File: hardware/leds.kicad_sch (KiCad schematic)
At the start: 4 parts, among them J21 USB_C_Receptacle_USB2.0_16P

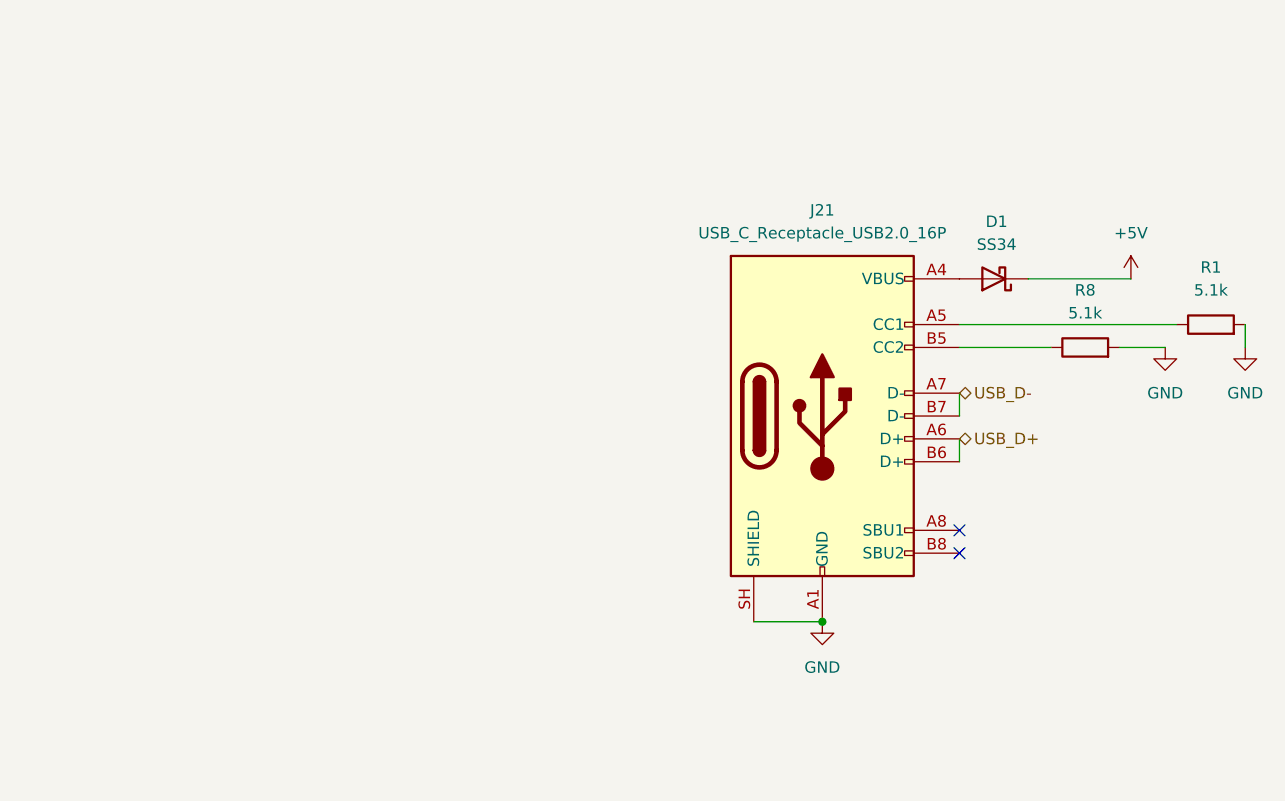
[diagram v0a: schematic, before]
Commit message: make the schematics
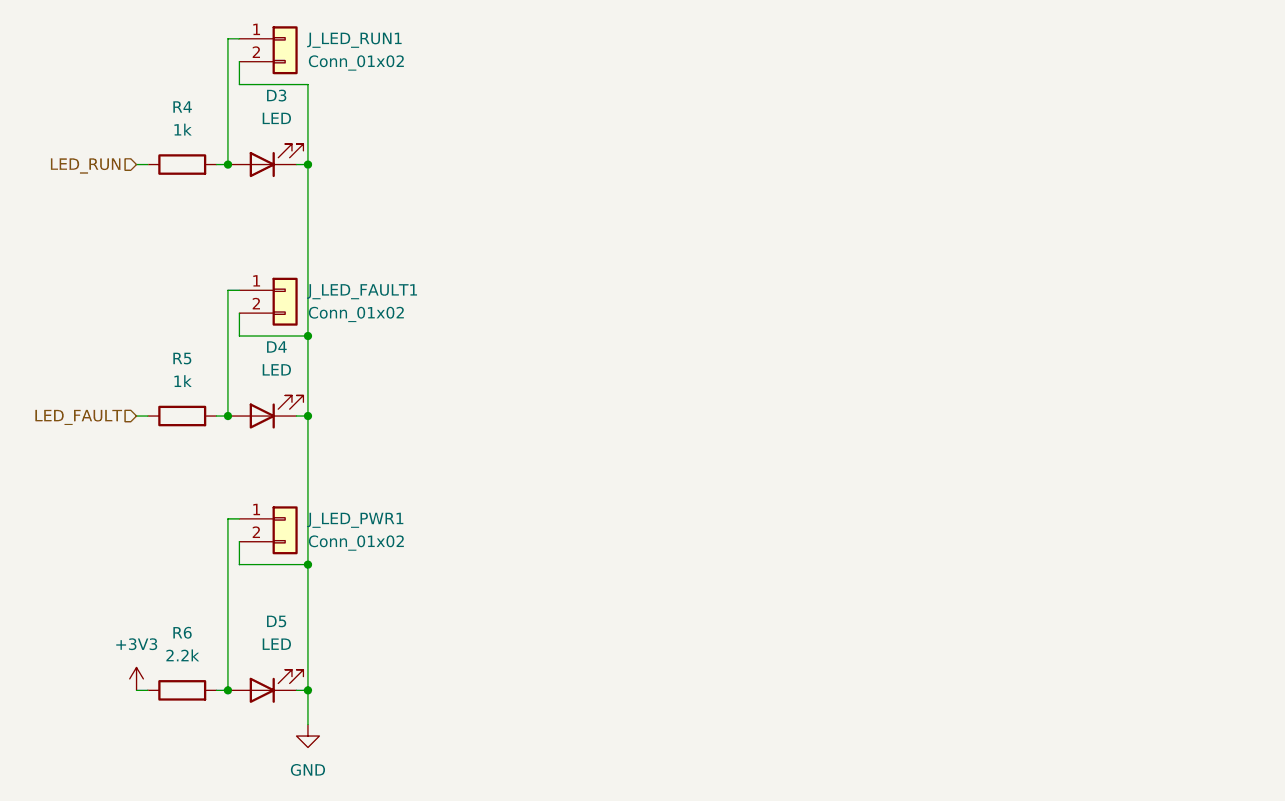
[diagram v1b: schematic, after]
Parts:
- removed D1: SS34, Diode_SMD:D_SMA, symbol Device:D_Schottky
- removed J21: USB_C_Receptacle_USB2.0_16P, symbol Connector:USB_C_Receptacle_USB2.0_16P
- removed R1, R8: 5.1k, symbol Device:R
- added D3, D4, D5: LED, symbol Device:LED
- added J_LED_FAULT1, J_LED_PWR1, J_LED_RUN1: Conn_01x02, symbol Connector_Generic:Conn_01x02
- added R4, R5: 1k, symbol Device:R
- added R6: 2.2k, symbol Device:R
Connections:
- net GND: now also D3.1 (K), D4.1 (K), D5.1 (K), J_LED_FAULT1.2 (Pin_2), J_LED_PWR1.2 (Pin_2), J_LED_RUN1.2 (Pin_2)
- new net: D4.2 (A), J_LED_FAULT1.1 (Pin_1), R5.2
- new net: D3.2 (A), J_LED_RUN1.1 (Pin_1), R4.2
- new net: D5.2 (A), J_LED_PWR1.1 (Pin_1), R6.2
- new net +3V3: R6.1
- new net LED_FAULT: R5.1
- new net LED_RUN: R4.1
- no-connect marks 2 -> 0

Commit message: place the stuff on the pcb
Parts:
- D3, D4, D5: footprint (none) -> LED_SMD:LED_2512_6332Metric
- J_LED_FAULT1, J_LED_PWR1, J_LED_RUN1: footprint (none) -> Connector_JST:JST_PH_B2B-PH-K_1x02_P2.00mm_Vertical
- R4, R5, R6: footprint (none) -> PCM_JLCPCB:R_0603
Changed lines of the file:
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@@
 			)
 		)
-		(property "Footprint" ""
+		(property "Footprint" "LED_SMD:LED_2512_6332Metric"
 			(at 53.34 74.93 0)
 			(hide yes)
@@
 			)
 		)
-		(property "Footprint" ""
+		(property "Footprint" "Connector_JST:JST_PH_B2B-PH-K_1x02_P2.00mm_Vertical"
 			(at 55.88 60.96 0)
 			(hide yes)
@@
 			)
 		)
-		(property "Footprint" ""
+		(property "Footprint" "PCM_JLCPCB:R_0603"
 			(at 44.45 76.708 90)
 			(hide yes)
@@
 			)
 		)
-		(property "Footprint" ""
+		(property "Footprint" "PCM_JLCPCB:R_0603"
 			(at 44.45 48.768 90)
 			(hide yes)
@@
 			)
 		)
-		(property "Footprint" ""
+		(property "Footprint" "PCM_JLCPCB:R_0603"
 			(at 44.45 107.188 90)
 			(hide yes)
@@
 			)
 		)
-		(property "Footprint" ""
+		(property "Footprint" "Connector_JST:JST_PH_B2B-PH-K_1x02_P2.00mm_Vertical"
 			(at 55.88 33.02 0)
 			(hide yes)
@@
 			)
 		)
-		(property "Footprint" ""
+		(property "Footprint" "LED_SMD:LED_2512_6332Metric"
 			(at 53.34 46.99 0)
 			(hide yes)
@@
 			)
 		)
-		(property "Footprint" ""
+		(property "Footprint" "LED_SMD:LED_2512_6332Metric"
 			(at 53.34 105.41 0)
 			(hide yes)
@@
 			)
 		)
-		(property "Footprint" ""
+		(property "Footprint" "Connector_JST:JST_PH_B2B-PH-K_1x02_P2.00mm_Vertical"
 			(at 55.88 86.36 0)
 			(hide yes)

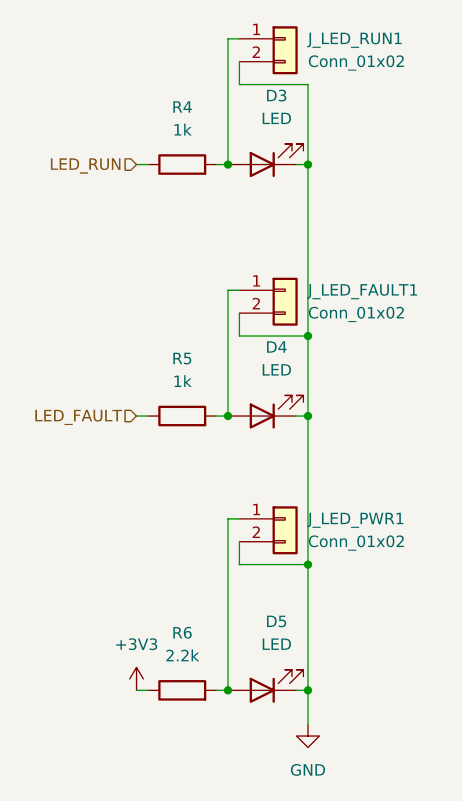
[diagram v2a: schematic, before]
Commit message: route
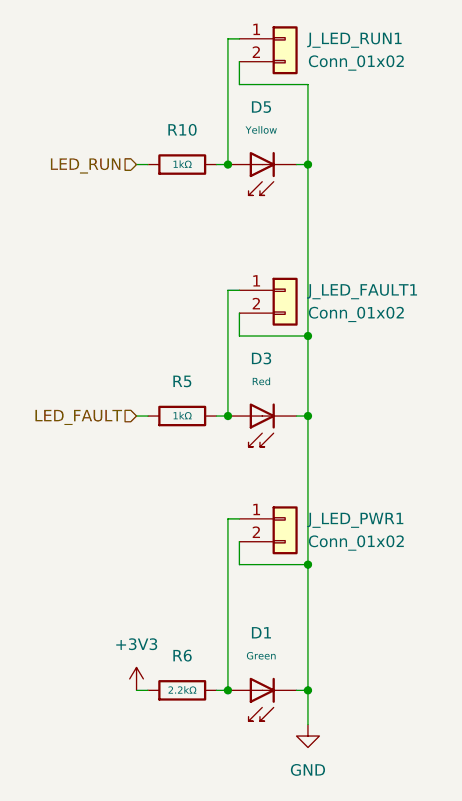
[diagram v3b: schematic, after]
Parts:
- removed D3, D4, D5: LED, LED_SMD:LED_2512_6332Metric, symbol Device:LED
- removed R4, R5: 1k, PCM_JLCPCB:R_0603, symbol Device:R
- removed R6: 2.2k, PCM_JLCPCB:R_0603, symbol Device:R
- added D1: Green, PCM_JLCPCB:D_0805, symbol PCM_JLCPCB-Diodes:LED,0805,Green
- added D3: Red, PCM_JLCPCB:D_0603, symbol PCM_JLCPCB-Diodes:LED,0603,Red
- added D5: Yellow, PCM_JLCPCB:D_0603, symbol PCM_JLCPCB-Diodes:LED,0603,Yellow
- added R10, R5: 1kΩ, PCM_JLCPCB:R_0603, symbol PCM_JLCPCB-Resistors:0603,1kΩ
- added R6: 2.2kΩ, PCM_JLCPCB:R_0603, symbol PCM_JLCPCB-Resistors:0603,2.2kΩ
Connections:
- net +3V3: now also R6.1
- net GND: now also D1.1, D3.1, D5.1
- net LED_FAULT: now also R5.1
- net LED_RUN: now also R10.1
- net at J_LED_FAULT1.1 (Pin_1): now also D3.2, R5.2
- net at J_LED_RUN1.1 (Pin_1): now also D5.2, R10.2
- net at J_LED_PWR1.1 (Pin_1): now also D1.2, R6.2
